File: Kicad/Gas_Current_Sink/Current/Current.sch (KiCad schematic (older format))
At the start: 5 parts, among them J1 CONN_01X04

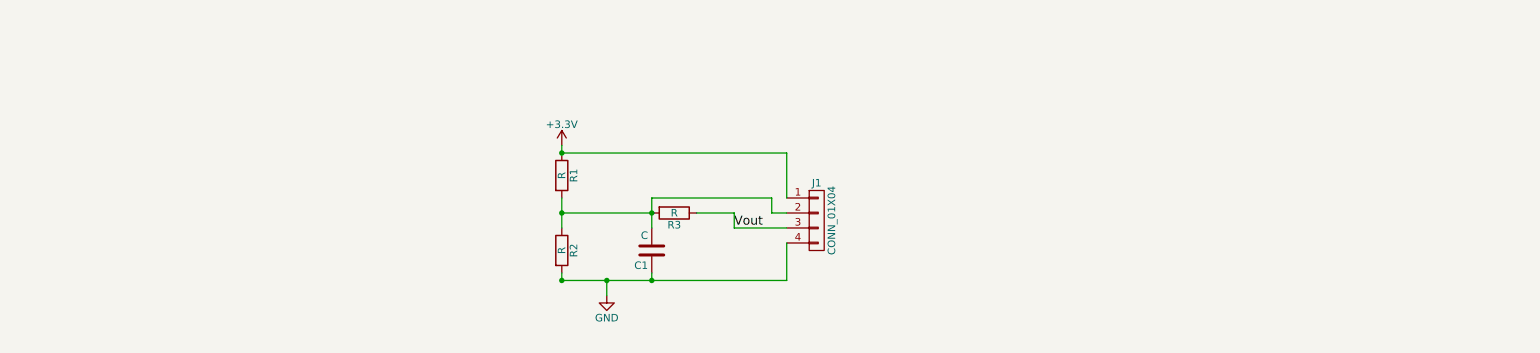
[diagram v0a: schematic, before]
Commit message: dimensionamento cs
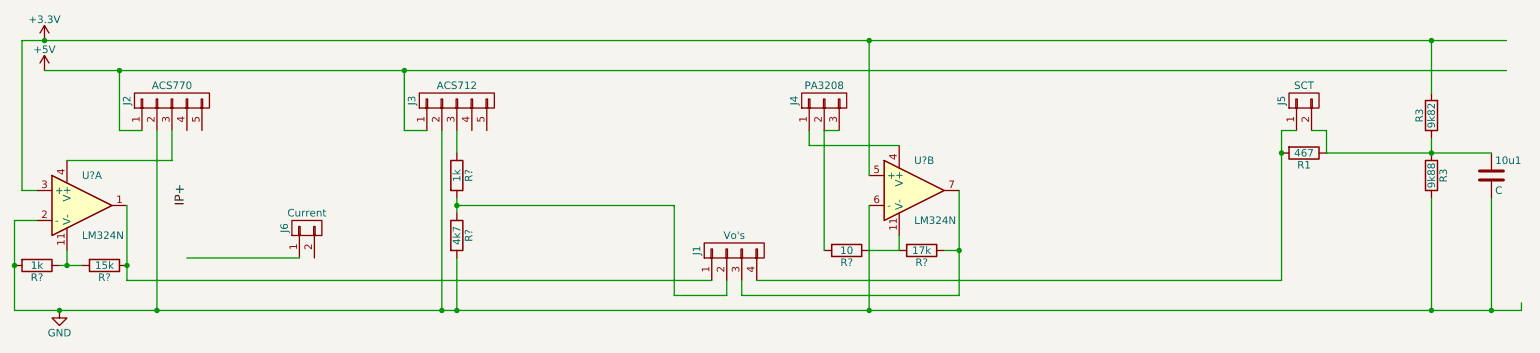
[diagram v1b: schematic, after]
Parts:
- removed C1: C, symbol C
- removed R2, R3: R, symbol R
- added 10u1: C, symbol C
- added J2: ACS770, symbol CONN_01X05
- added J3: ACS712, symbol CONN_01X05
- added J4: PA3208, symbol CONN_01X03
- added J5: SCT, symbol CONN_01X02
- added J6: Current, symbol CONN_01X02
- added R3: 9k82, symbol R
- added R3: 9k88, symbol R
- added R? (x2): 1k, symbol R
- added R?: 4k7, symbol R
- added R?: 15k, symbol R
- added R?: 10, symbol R
- added R?: 17k, symbol R
- added U? (x2): LM324N, symbol LM324N
- J1: value CONN_01X04 -> Vo's
- R1: value R -> 467
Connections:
- net labels added: +5V, IP+
- net labels removed: Vout
- wire segments 17 -> 50
